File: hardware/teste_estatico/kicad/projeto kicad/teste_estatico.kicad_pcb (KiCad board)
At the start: 2 copper layers, 92.1 x 81.2 mm, 11 parts, among them J1 PINHD_1x6_Female, J2 PINHD_1x2_Female

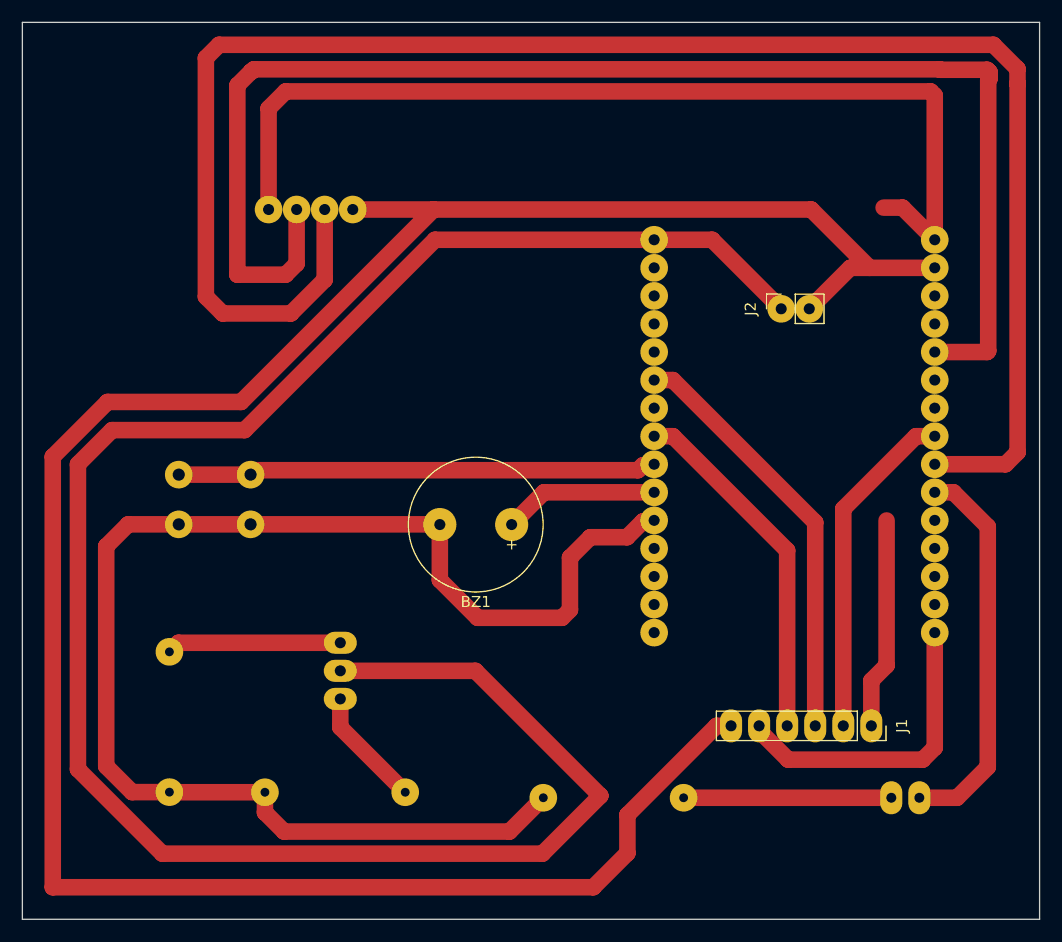
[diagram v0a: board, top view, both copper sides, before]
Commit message: chore: atualizando a pcb
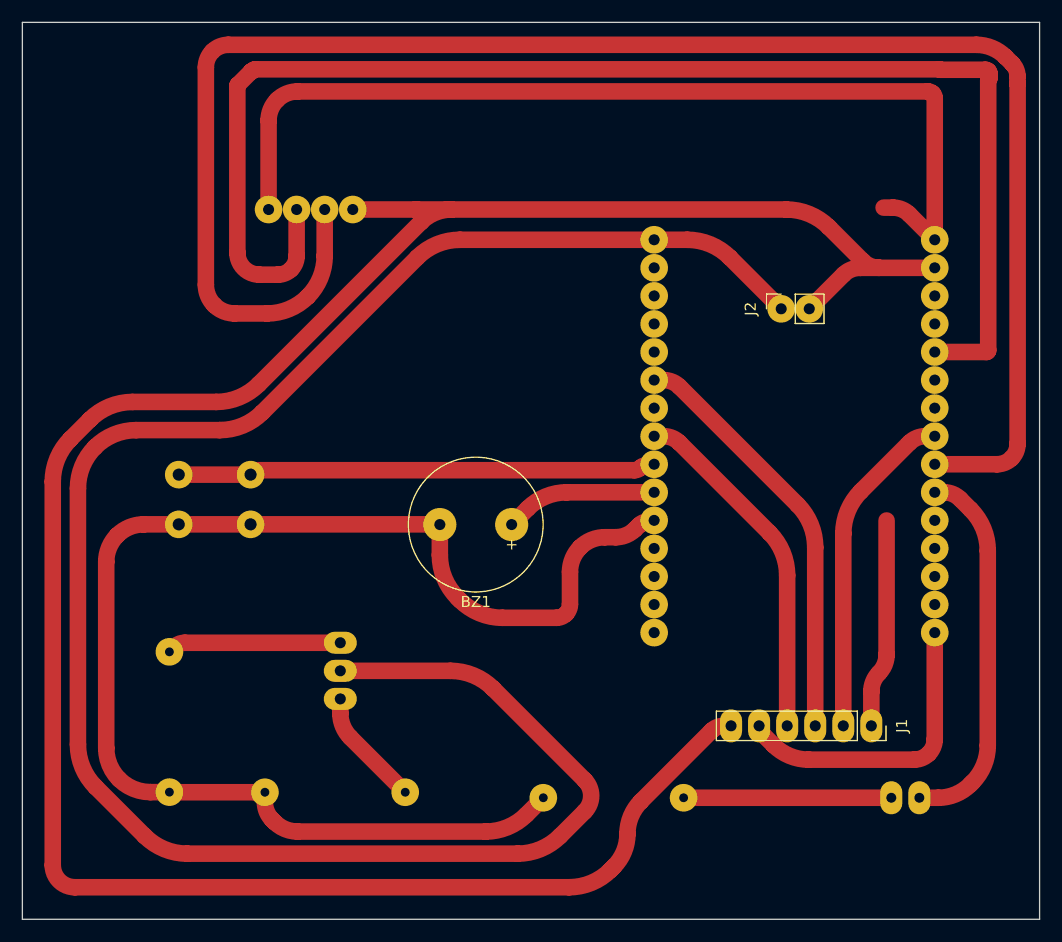
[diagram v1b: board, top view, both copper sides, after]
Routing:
- net VIN: track 183.1 -> 179.8 mm
- net Net-(A1-ADC1_CH7/D35): track 127.6 -> 124.8 mm
- net GND: track 214.1 -> 215.7 mm
- net Net-(A1-D18): track 158.1 -> 156.8 mm
- net Net-(A1-D4/ADC2_CH0): track 126.8 -> 125.6 mm
- net Net-(A1-D19): track 35.2 -> 34.4 mm
- net 3.3V: track 108.3 -> 107.7 mm
